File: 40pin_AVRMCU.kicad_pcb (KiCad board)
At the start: 2 copper layers, 25.4 x 52.1 mm, 21 parts, among them IC1 ATMEGA32-A, P1 CONN_5X2, P2 CONN_10, P3 CONN_10, P4 CONN_10, P5 CONN_10, P6 CONN_7, P7 CONN_01X01, SW1 rst, X1 16Mhz

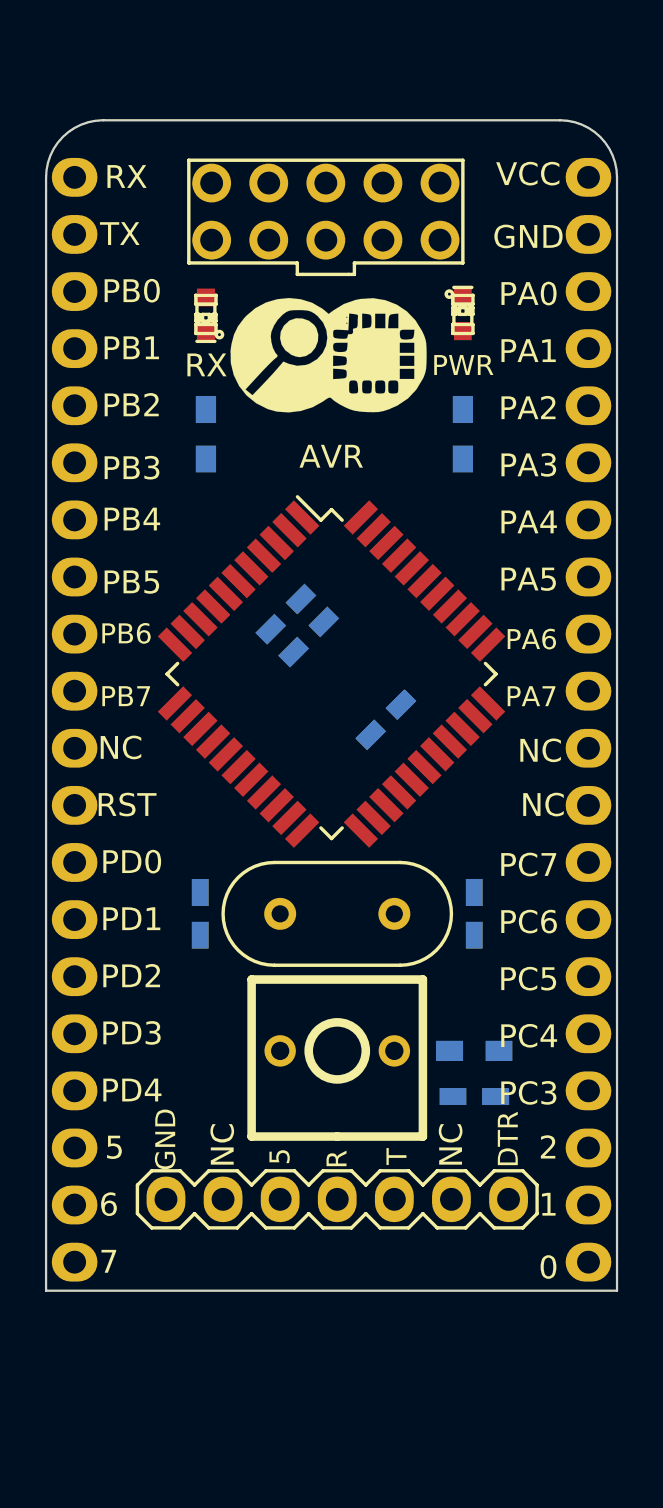
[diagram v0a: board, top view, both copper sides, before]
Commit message: Updated designs
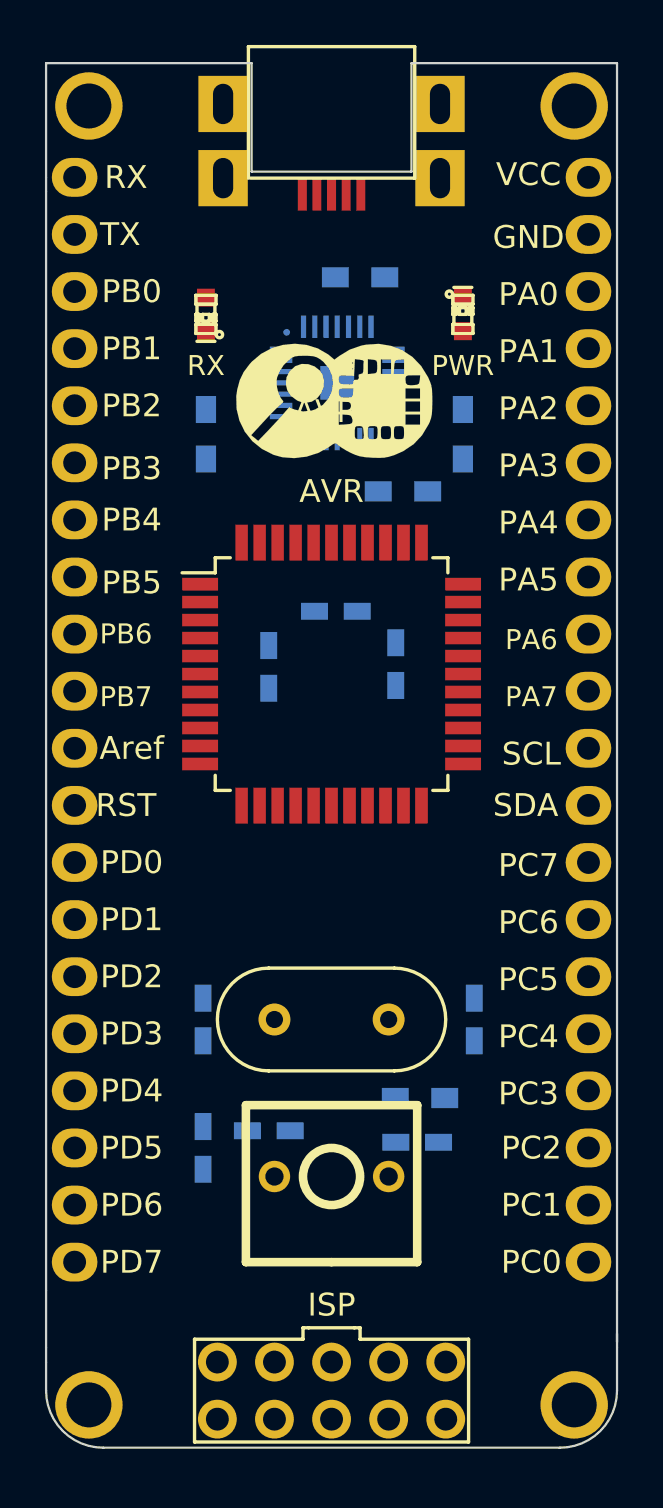
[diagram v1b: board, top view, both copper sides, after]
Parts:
- removed C1: 0.1uF, Capacitors_SMD:C_0603_HandSoldering
- added C7: 0.1uF, Capacitors_SMD:C_0603_HandSoldering, B.Cu at (194.1, 152.9)
- added C8: 0.1uF, Capacitors_SMD:C_0603_HandSoldering, B.Cu at (191.1, 153.7)
- added C9: 0.1uF, Capacitors_SMD:C_0603_HandSoldering, B.Cu at (200.7, 153.4)
- added CON1: USB-MINI-B, EE:USB_Micro-B_SMD_NEW, F.Cu at (196.8, 111.1)
- added P10: CONN_01X01, Connect:1pin, F.Cu at (207.6, 107.3)
- added P8: CONN_01X01, Connect:1pin, F.Cu at (207.6, 165.1)
- added P9: CONN_01X01, Connect:1pin, F.Cu at (186.1, 107.3)
- added R4: R, Resistors_SMD:R_0603_HandSoldering, B.Cu at (198.1, 114.9)
- added R5: R, Resistors_SMD:R_0603_HandSoldering, B.Cu at (200.0, 124.5)
- added U1: CP2102, EE:cp2102_xl2, B.Cu at (197.1, 119.6)
- P6: value CONN_7 -> CONN_01X01; footprint Pin_Headers:Pin_Header_Straight_1x07 -> Connect:1pin
- moved P1 51.0 mm to (201.9, 163.2), turned to 270 degrees
- moved C2 13.1 mm to (203.2, 148.0), turned to 270 degrees
- moved C3 12.9 mm to (191.1, 148.0), turned to 90 degrees
- moved P6 9.77 mm to (186.1, 165.1), turned to 0 degrees
- moved X1 7.11 mm to (194.3, 148.0), turned to 0 degrees
- moved C6 5.71 mm to (194.1, 132.3), turned to 270 degrees
- moved SW1 5.59 mm to (196.8, 154.9)
- moved C4 5.37 mm to (199.7, 132.1), turned to 270 degrees
- moved R1 3.20 mm to (200.8, 151.4)
- moved P7 2.05 mm to (196.8, 120.4)
- moved C5 1.66 mm to (197.0, 129.8), turned to 180 degrees
- turned IC1 to 0 degrees
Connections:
- C4 pad 1: /+5V -> /Aref
- IC1 pad 19: Net-(IC1-Pad19) -> /SCL
- IC1 pad 20: Net-(IC1-Pad20) -> /SDA
- IC1 pad 29: /+5V -> /Aref
- P2 pad 1: Net-(P2-Pad1) -> /Aref
- P4 pad 1: Net-(IC1-Pad19) -> /SCL
- P4 pad 10: Net-(P4-Pad10) -> /SCL
- P4 pad 2: Net-(IC1-Pad20) -> /SDA
- P4 pad 9: Net-(P4-Pad9) -> /SDA
- P6 pad 1: GND -> Net-(P6-Pad1)
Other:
- board size 25.4 x 52.1 mm -> 25.4 x 61.6 mm
- net class Default: clearance 0.254 -> 0.1651
- rule trace_clearance: 0.254 -> 0.1651
- board text added: "."
- board text added: "Aref"
- board text added: "Atmega16 Atmega32"
- board text added: "ISP"
- board text added: "PC0"
- board text added: "PC1"
- board text added: "PC2"
- board text added: "PD5"
- board text added: "PD6"
- board text added: "PD7"
- board text added: "SCL"
- board text added: "SDA"
- board text removed: "0"
- board text removed: "1"
- board text removed: "2"
- board text removed: "5"
- board text removed: "6"
- board text removed: "7"
- board text removed: "DTR"
- board text removed: "NC"
- board text removed: "R"
- board text removed: "T"

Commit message: updated
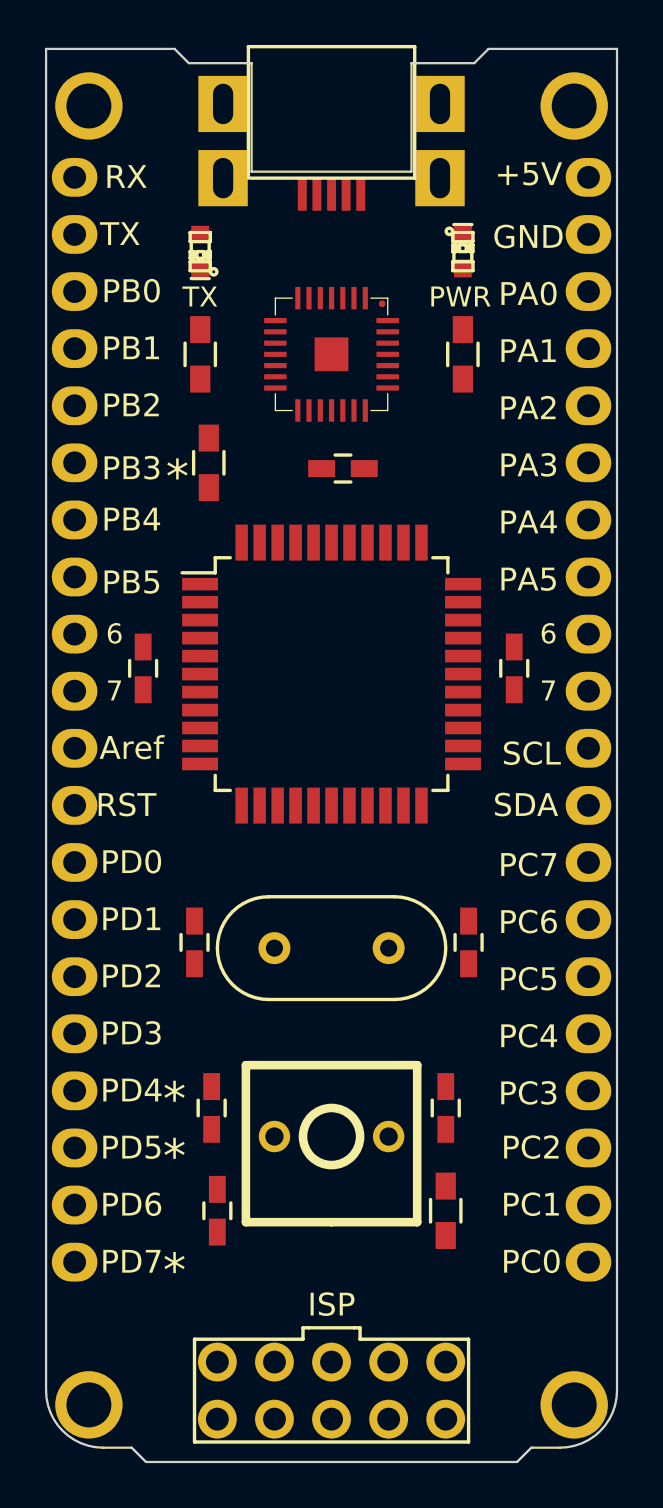
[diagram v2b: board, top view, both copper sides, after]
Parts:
- removed R4: R, Resistors_SMD:R_0603_HandSoldering
- C2, C3, C4, C5, C6, C7, C8, C9, R1, R2, R3, U1: moved to F.Cu
- P7: moved to B.Cu
- R5: value R -> 470; moved to F.Cu
- moved R5 8.73 mm to (191.4, 123.2), turned to 90 degrees
- moved C5 6.36 mm to (197.4, 123.4)
- moved C6 5.59 mm to (188.5, 132.3)
- moved P7 5.33 mm to (196.8, 125.7), turned to 270 degrees
- moved C4 5.27 mm to (205.0, 132.3)
- moved R1 5.15 mm to (201.9, 156.5), turned to 270 degrees
- moved C7 4.23 mm to (191.8, 156.5), turned to 270 degrees
- moved R3 3.57 mm to (191.0, 118.4)
- moved R2 3.56 mm to (202.7, 118.4)
- moved C3 3.45 mm to (190.8, 144.5), turned to 270 degrees
- moved C2 3.44 mm to (202.9, 144.5)
- moved X1 3.18 mm to (194.3, 144.8)
- moved D3 2.81 mm to (191.0, 113.8)
- moved D1 2.79 mm to (202.7, 113.8)
- moved C9 1.98 mm to (201.9, 151.9), turned to 90 degrees
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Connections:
- CON1 pad 5: Net-(CON1-Pad5) -> GND
- U1 pad 25: Net-(R4-Pad2) -> /TX
- U1 pad 3: Net-(CON1-Pad4) -> GND
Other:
- board size 25.4 x 61.6 mm -> 25.4 x 62.9 mm
- board text added: "*"
- board text added: "+5V"
- board text added: "6"
- board text added: "7"
- board text added: "ExploreEmbedded.com"
- board text added: "PWM *"
- board text removed: "AVR"
- board text removed: "PA6"
- board text removed: "PA7"
- board text removed: "PB6"
- board text removed: "PB7"
- board text removed: "VCC"
